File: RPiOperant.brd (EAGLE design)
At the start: 136 x 100 mm, 69 parts, among them IC1 74LS14N, IC2 74LS14N, J2 POWER_JACK, J3 POWER_JACK

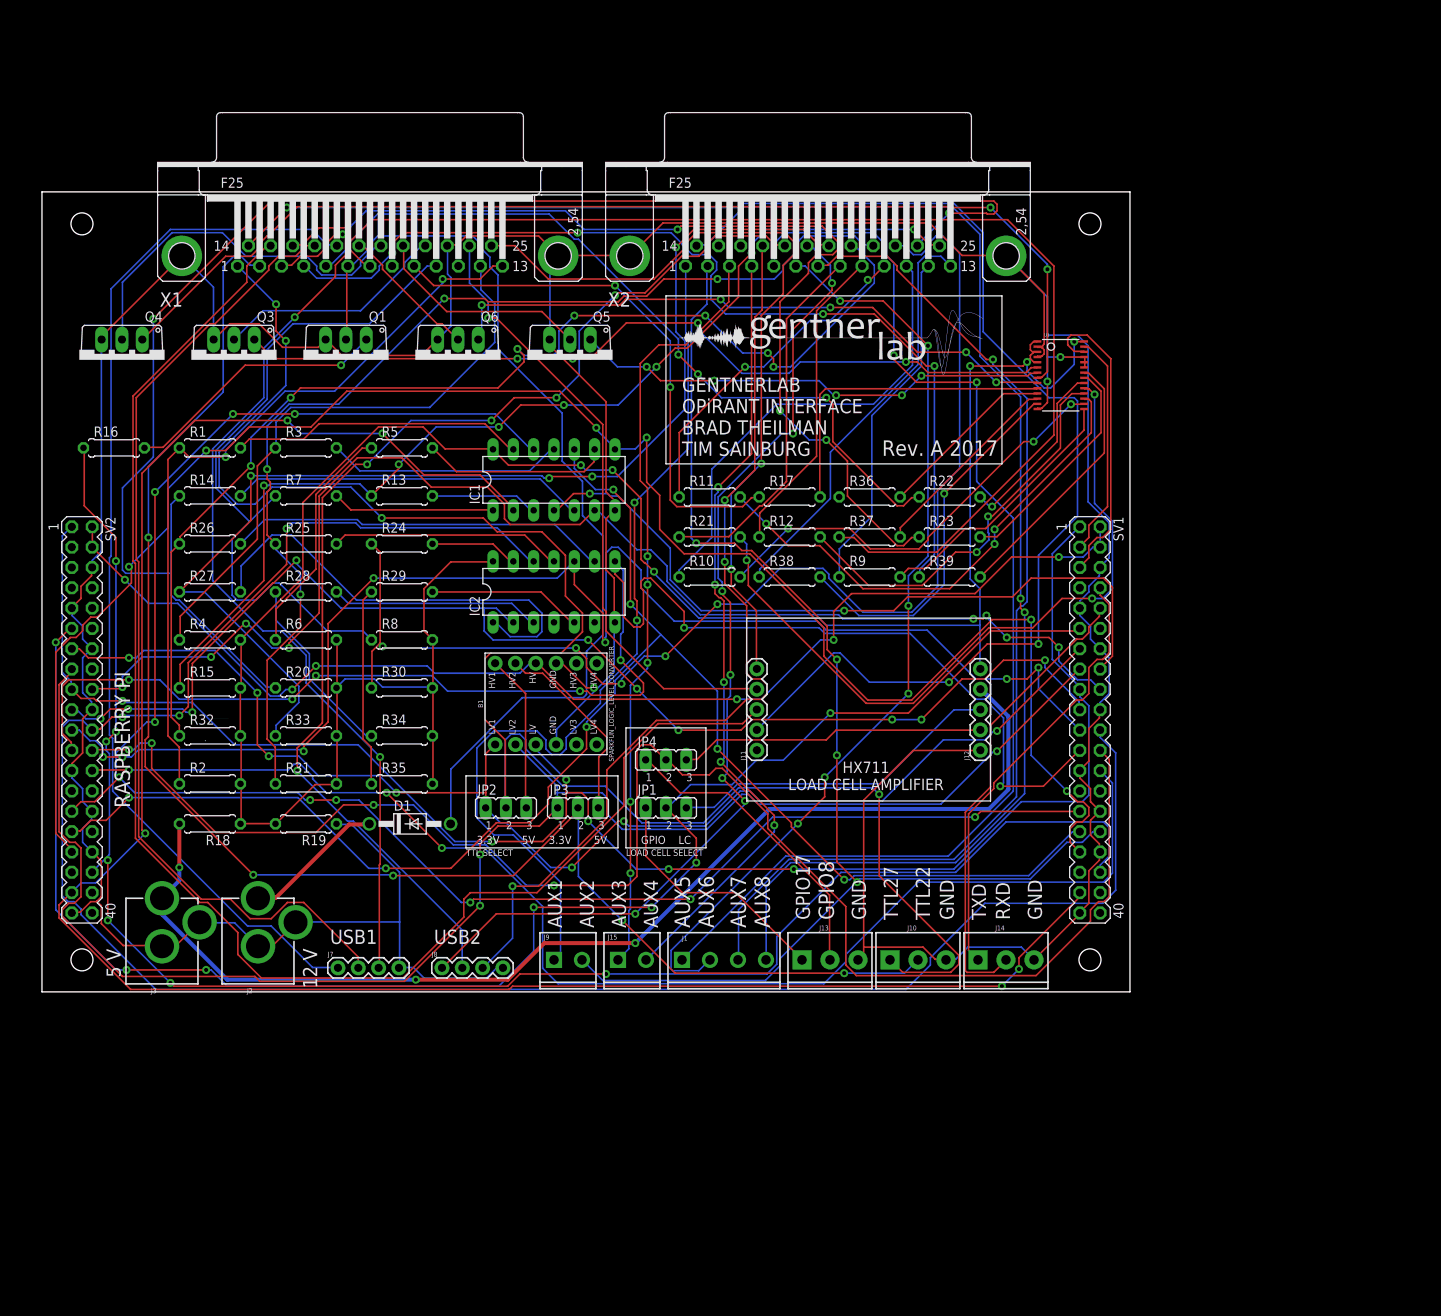
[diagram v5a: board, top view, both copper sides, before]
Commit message: revision b
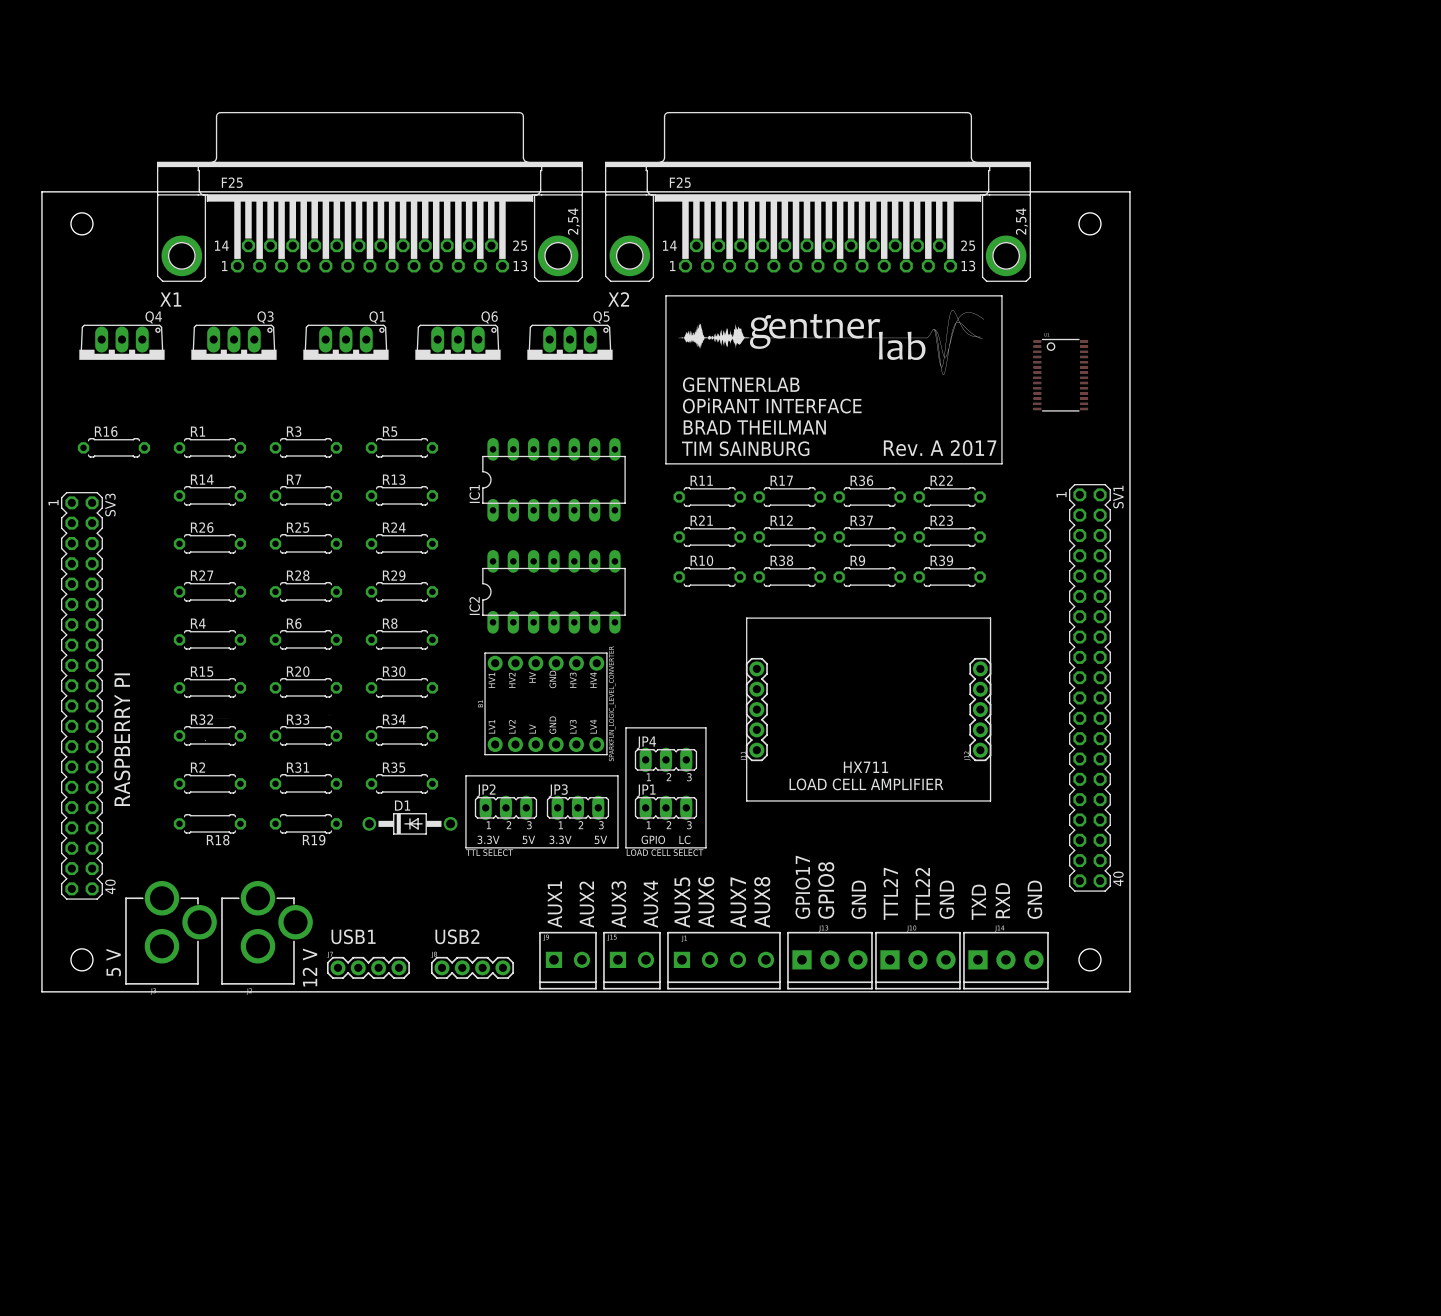
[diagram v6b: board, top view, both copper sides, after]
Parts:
- removed SV2: (no value), con-lstb:MA20-2
- added SV3: (no value), con-lstb:MA20-2
- moved SV1 4.00 mm to (131.0, 38.0)
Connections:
- removed net CENTNER_IR: R5.1, R6.1
- new net GPIO4: SV1.7, SV3.7
- new net ID_SC: SV1.28, SV3.28
- new net ID_SD: SV1.27, SV3.27
- new net PCM_CLK: SV1.12, SV3.12
- new net PCM_DIN: SV1.38, SV3.38
- new net PCM_DOUT: SV1.40, SV3.40
- new net PCM_FS: SV1.35, SV3.35
- net AUX2: now also SV3.32
- net CENTER_IR: now also R5.1, R6.1
- net CENTER_PECK_GPIO: now also SV3.33; no longer SV2.33
- net GND: now also SV3.14, SV3.20, SV3.25, SV3.30, SV3.34, SV3.39, SV3.6, SV3.9; no longer SV2.14, SV2.20, SV2.25, SV2.30, SV2.34, SV2.39, SV2.6, SV2.9
- net GPIO17: now also SV3.11; no longer SV2.11
- net GPIO22: now also SV3.15; no longer SV2.15
- net GPIO27: now also SV3.13; no longer SV2.13
- net GPIO7: now also SV3.26; no longer SV2.26
- net GPIO8: now also SV3.24; no longer SV2.24
- net HOPPER_IR_GPIO: now also SV3.29; no longer SV2.29
- net HOPPER_TRIG_GPIO: now also SV3.36; no longer SV2.36
- net IR_1_GPIO: now also SV3.16
- net IR_2_GPIO: now also SV3.18; no longer SV2.18
- net IR_3_GPIO: now also SV3.22; no longer SV2.22
- net IR_4_GPIO: now also SV3.21; no longer SV2.21
- net IR_5_GPIO: now also SV3.23; no longer SV2.23
- net IR_6_GPIO: now also SV3.19; no longer SV2.19
- net LEFT_PECK_GPIO: now also SV3.31; no longer SV2.31
- net RIGHT_PECK_GPIO: now also SV3.37; no longer SV2.37
- net RPI_3.3V: now also SV3.1, SV3.17; no longer SV2.1, SV2.17
- net RPI_5V: now also SV3.2, SV3.4; no longer SV2.2, SV2.4
- net RXD: now also SV3.10
- net SCL: now also SV3.5
- net SDA: now also SV3.3
- net TXD: now also SV3.8
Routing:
- net GND: track 583.7 -> 0.00 mm, vias 3 -> 0
- net +3V3: track 291.8 -> 0.00 mm, vias 6 -> 0
- net IR_3_GPIO: track 262.9 -> 0.00 mm, vias 3 -> 0
- net RIGHT_PECK_GPIO: track 252.8 -> 0.00 mm, vias 5 -> 0
- net HOPPER_IR_GPIO: track 230.6 -> 0.00 mm, vias 10 -> 0
- net CENTER_PECK_GPIO: track 229.9 -> 0.00 mm, vias 6 -> 0
- net TTL27: track 223.9 -> 0.00 mm, vias 4 -> 0
- net RPI_3.3V: track 214.6 -> 0.00 mm, vias 6 -> 0
- net HOPPER_TRIG_GPIO: track 209.6 -> 0.00 mm, vias 7 -> 0
- net GPIO22: track 201.1 -> 0.00 mm, vias 3 -> 0
- net GPIO17: track 199.2 -> 0.00 mm, vias 7 -> 0
- net LOADCELLA-: track 198.4 -> 0.00 mm, vias 3 -> 0
- net GPIO8: track 197.8 -> 0.00 mm, vias 4 -> 0
- net LEFT_PECK_GPIO: track 196.4 -> 0.00 mm, vias 7 -> 0
- net IR_2: track 194.4 -> 0.00 mm, vias 2 -> 0
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
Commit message: updates
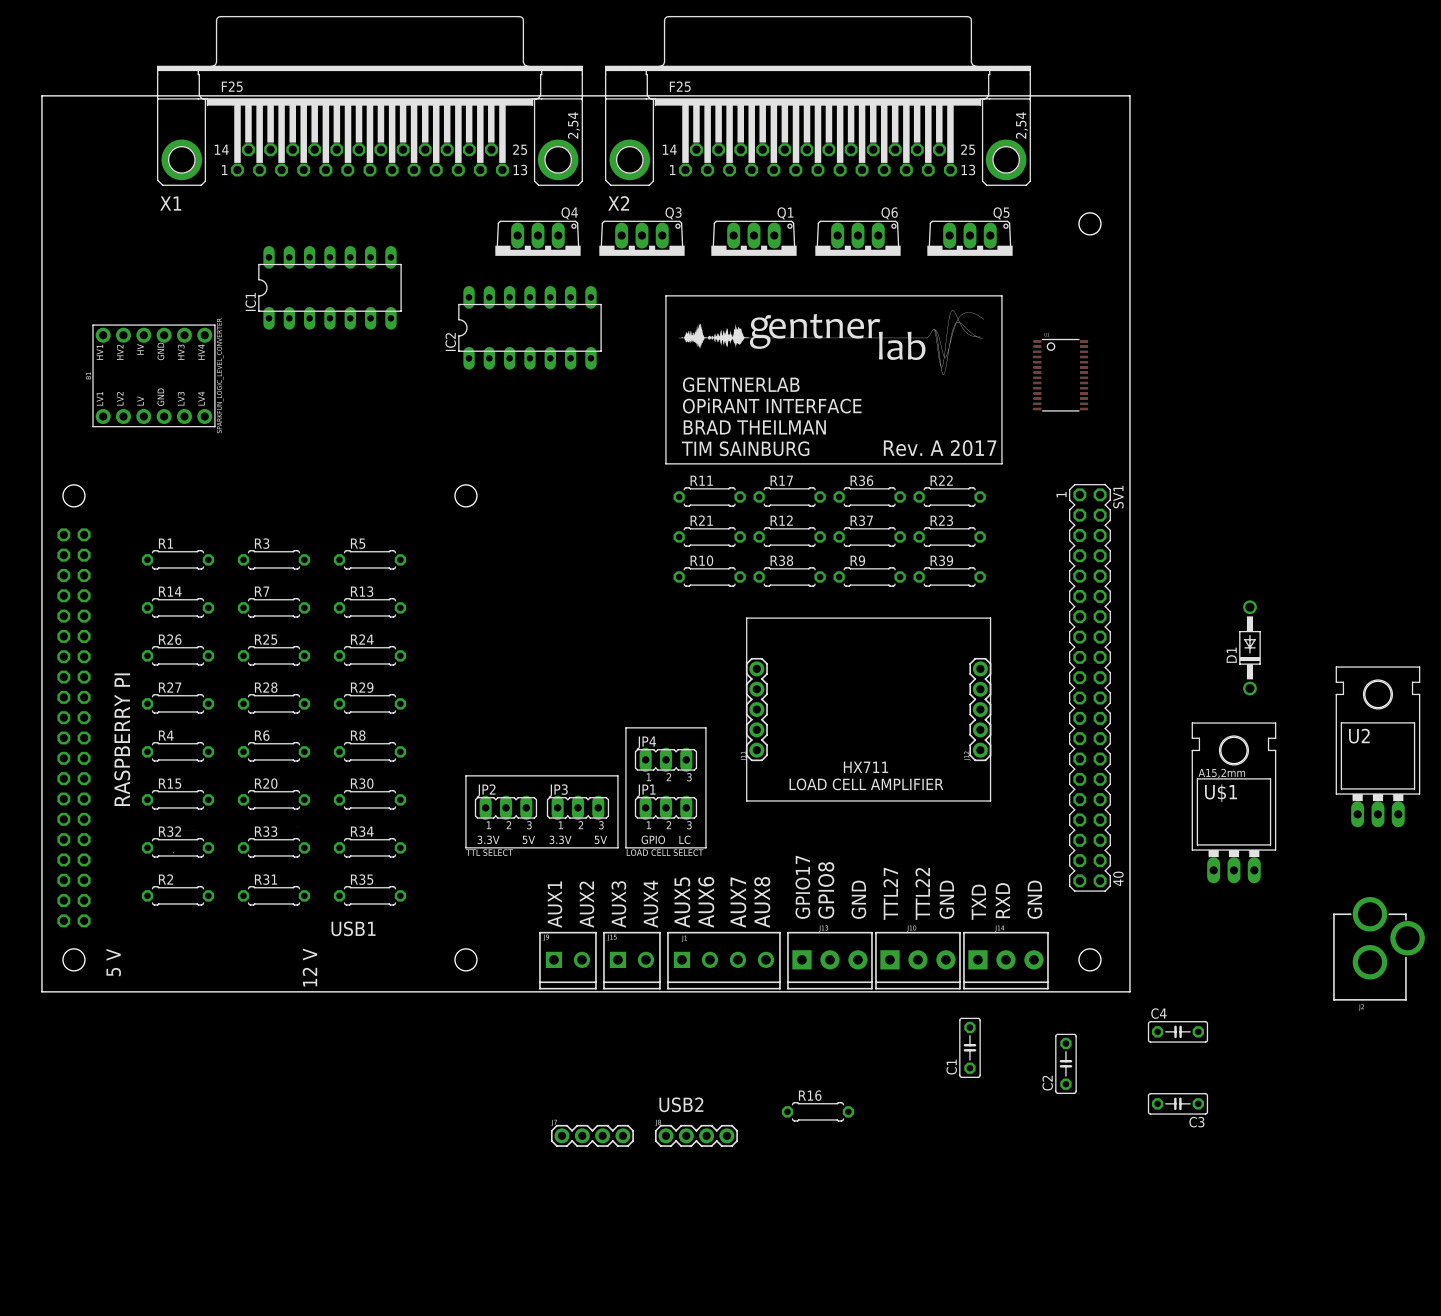
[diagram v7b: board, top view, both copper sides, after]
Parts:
- removed J3: POWER_JACK, SparkFun-Connectors:POWER_JACK_PTH
- removed R18: 10k, resistor:0207/7
- removed R19: 20k, resistor:0207/7
- added C1: 100nF, adafruit:C050-025X075
- added C2, C3, C4: 10uF, adafruit:C050-025X075
- added U$1: V_REG_LD1117VXX, SparkFun-IC-Power:78XXL
- added U2: (no value), SparkFun-IC-Power:TO-220-ALT
- moved J2 139.0 mm to (166.0, -4.00)
- moved R16 121.0 mm to (97.0, -15.0)
- moved D1 107.3 mm to (151.0, 43.0), turned to 90 degrees
- moved B1 63.9 mm to (14.0, 77.0)
- moved Q4 53.6 mm to (62.0, 92.0)
- moved Q1 52.6 mm to (89.0, 92.0)
- moved Q3 52.6 mm to (75.0, 92.0)
- moved Q5 51.7 mm to (116.0, 92.0)
- moved Q6 51.7 mm to (102.0, 92.0)
- moved IC1 36.9 mm to (36.0, 88.0)
- moved J7 35.0 mm to (65.0, -18.0)
- moved J8 35.0 mm to (78.0, -18.0)
- moved IC2 33.1 mm to (61.0, 83.0)
- moved R1 14.6 mm to (17.0, 54.0)
- moved R13 14.6 mm to (41.0, 48.0)
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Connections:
- new net 5V: C4.1, U2.OUT
- net +3V3: now also C2.1, U$1.GND; no longer R18.1, R19.2
- net +5V: no longer J3.PWR, R18.2
- net 12V: now also C1.1, C3.1, U$1.OUT, U2.IN
- net GND: now also C1.2, C2.2, C3.2, C4.2, U$1.IN, U2.GND; no longer J3.GND, J3.GNDBREAK, R19.1
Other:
- board size 136 x 100 mm -> 136 x 112 mm

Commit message: version 2
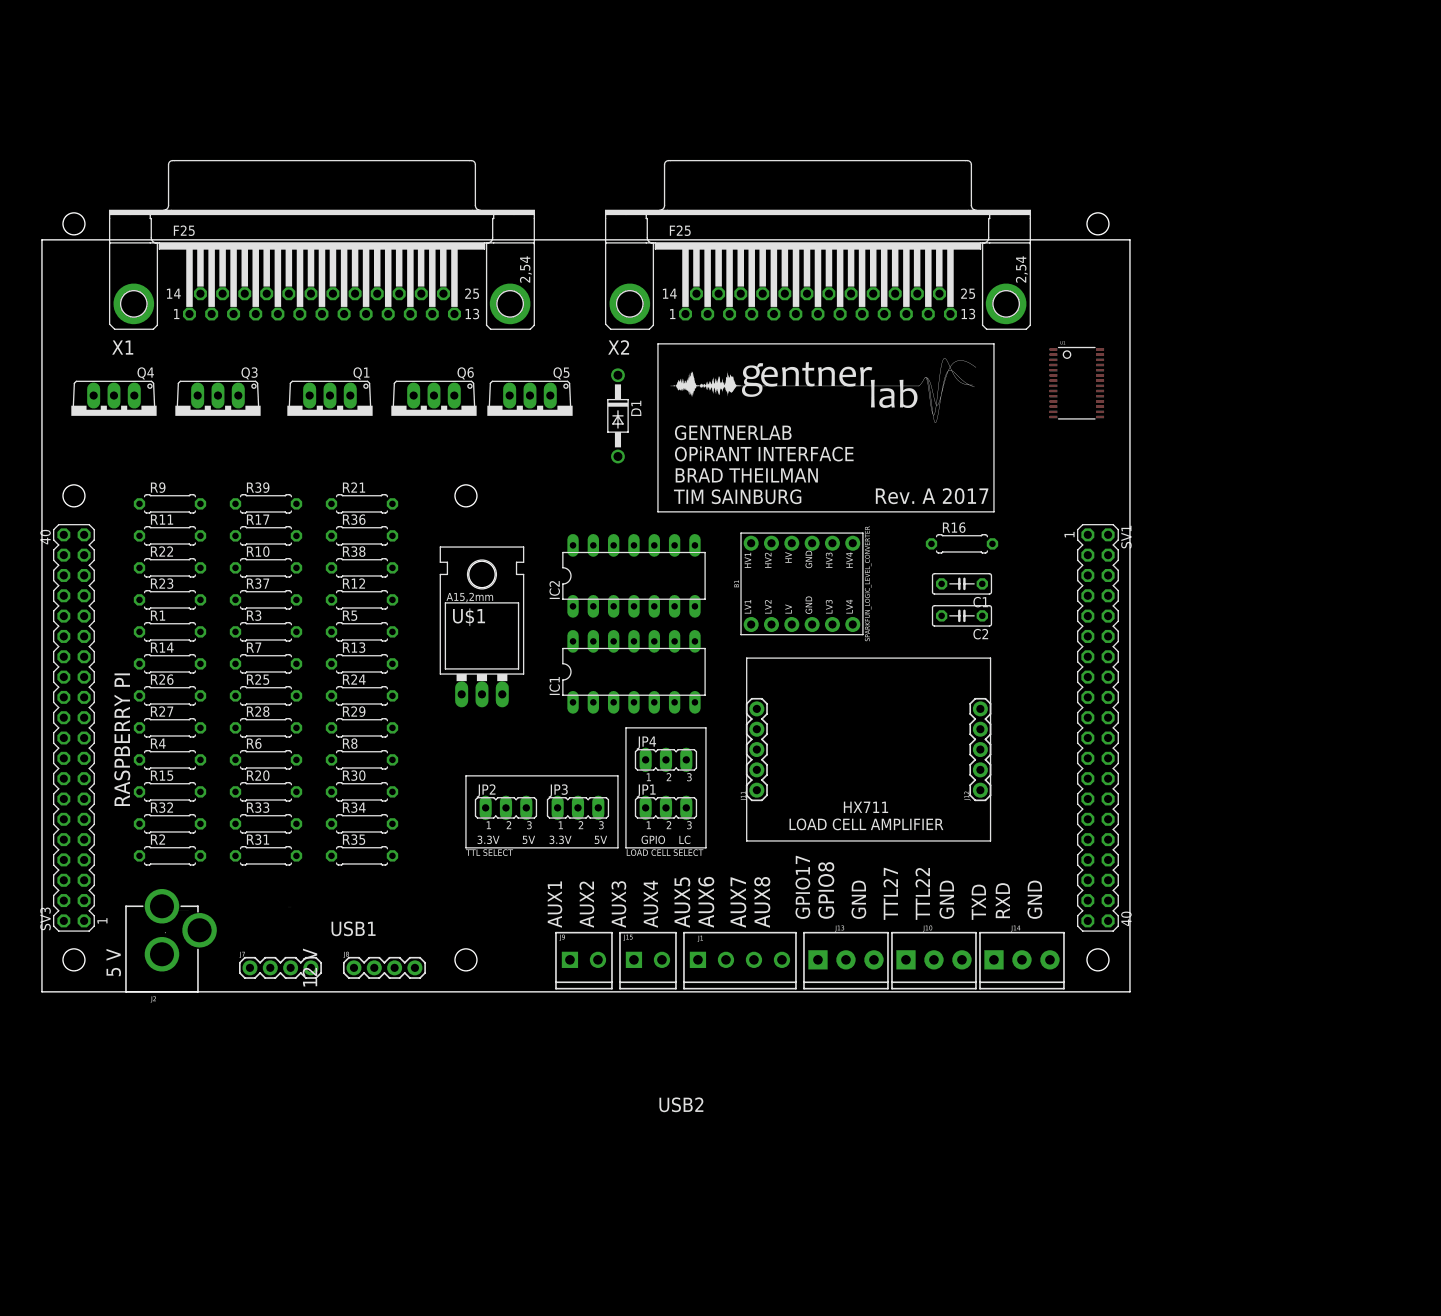
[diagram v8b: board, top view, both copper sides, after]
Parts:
- removed C3, C4: 10uF, adafruit:C050-025X075
- removed U2: (no value), SparkFun-IC-Power:TO-220-ALT
- moved J2 151.0 mm to (15.0, -3.00)
- moved R22 97.9 mm to (16.0, 53.0)
- moved R23 97.8 mm to (16.0, 49.0)
- moved U$1 96.5 mm to (55.0, 41.0)
- moved R9 87.9 mm to (16.0, 61.0)
- moved R39 85.9 mm to (28.0, 61.0)
- moved B1 85.1 mm to (95.0, 51.0)
- moved D1 84.2 mm to (72.0, 72.0), turned to 270 degrees
- moved R37 75.9 mm to (28.0, 49.0)
- moved R16 73.2 mm to (115.0, 56.0)
- moved R11 67.6 mm to (16.0, 57.0)
- moved R17 65.6 mm to (28.0, 57.0)
- moved R36 63.6 mm to (40.0, 57.0)
- moved IC1 61.2 mm to (74.0, 40.0)
- moved Q5 58.5 mm to (61.0, 72.0)
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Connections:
- removed net 5V: C4.1, U2.OUT
- net 12V: now also X1.23; no longer C3.1, U2.IN
- net GND: no longer C3.2, C4.2, U2.GND, X1.23
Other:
- board size 136 x 112 mm -> 136 x 94 mm
